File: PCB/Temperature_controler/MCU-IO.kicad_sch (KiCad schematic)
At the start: 14 parts, among them U1 STM32F401RBTx

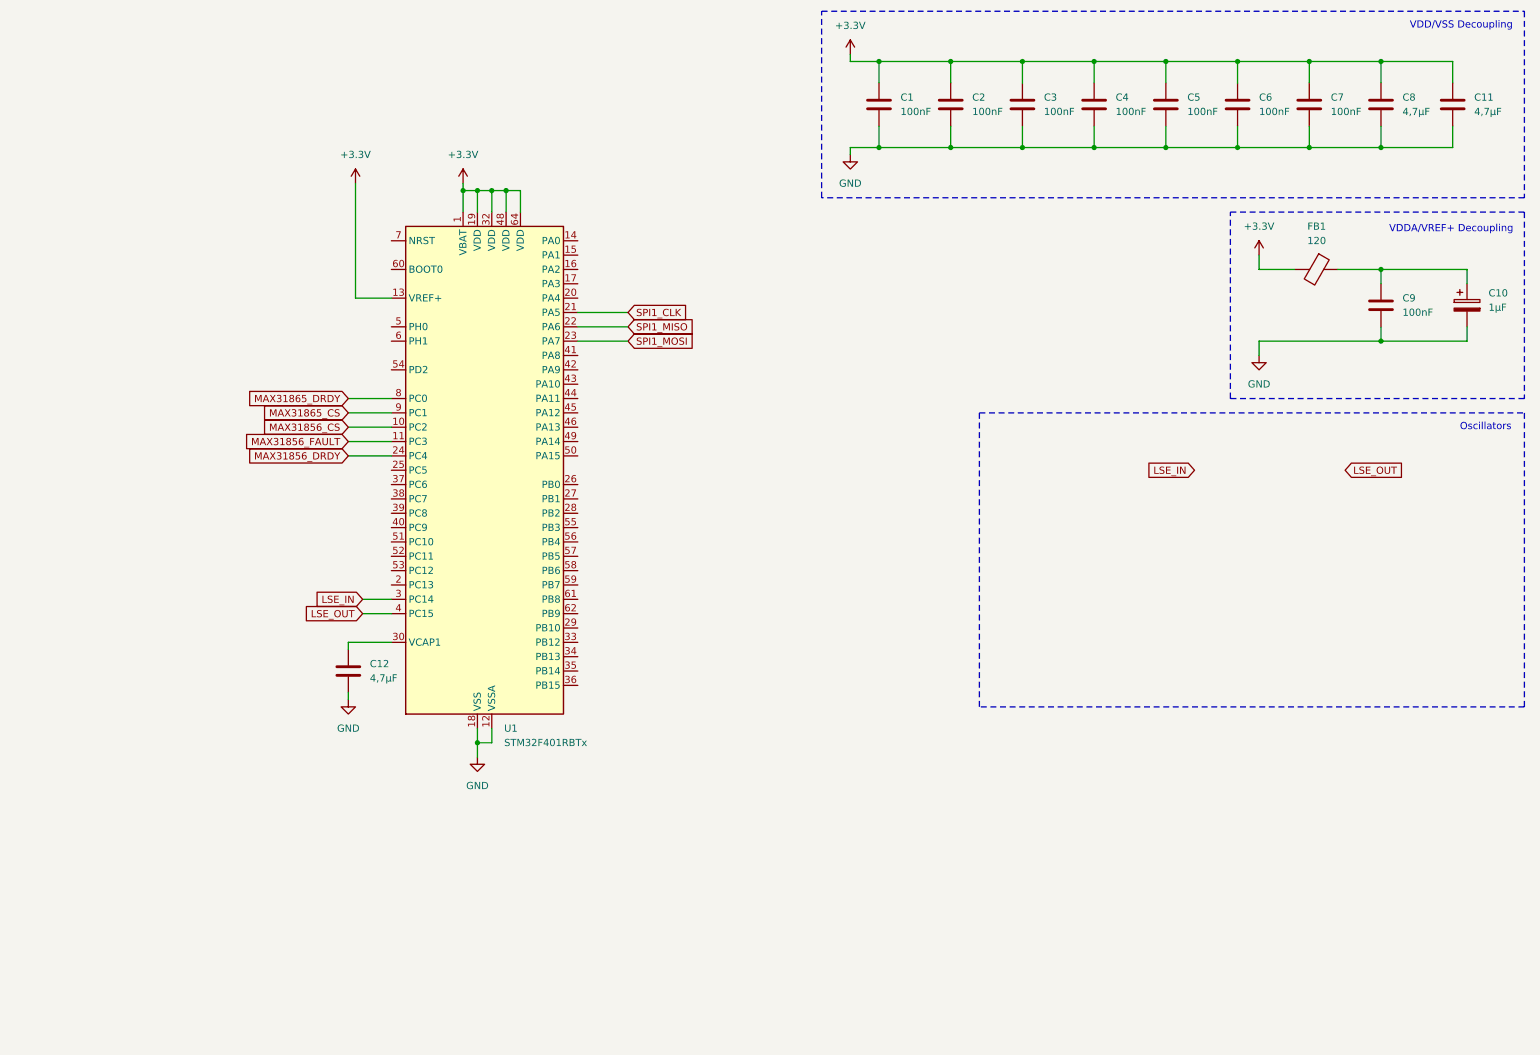
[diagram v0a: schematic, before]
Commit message: PCB progress
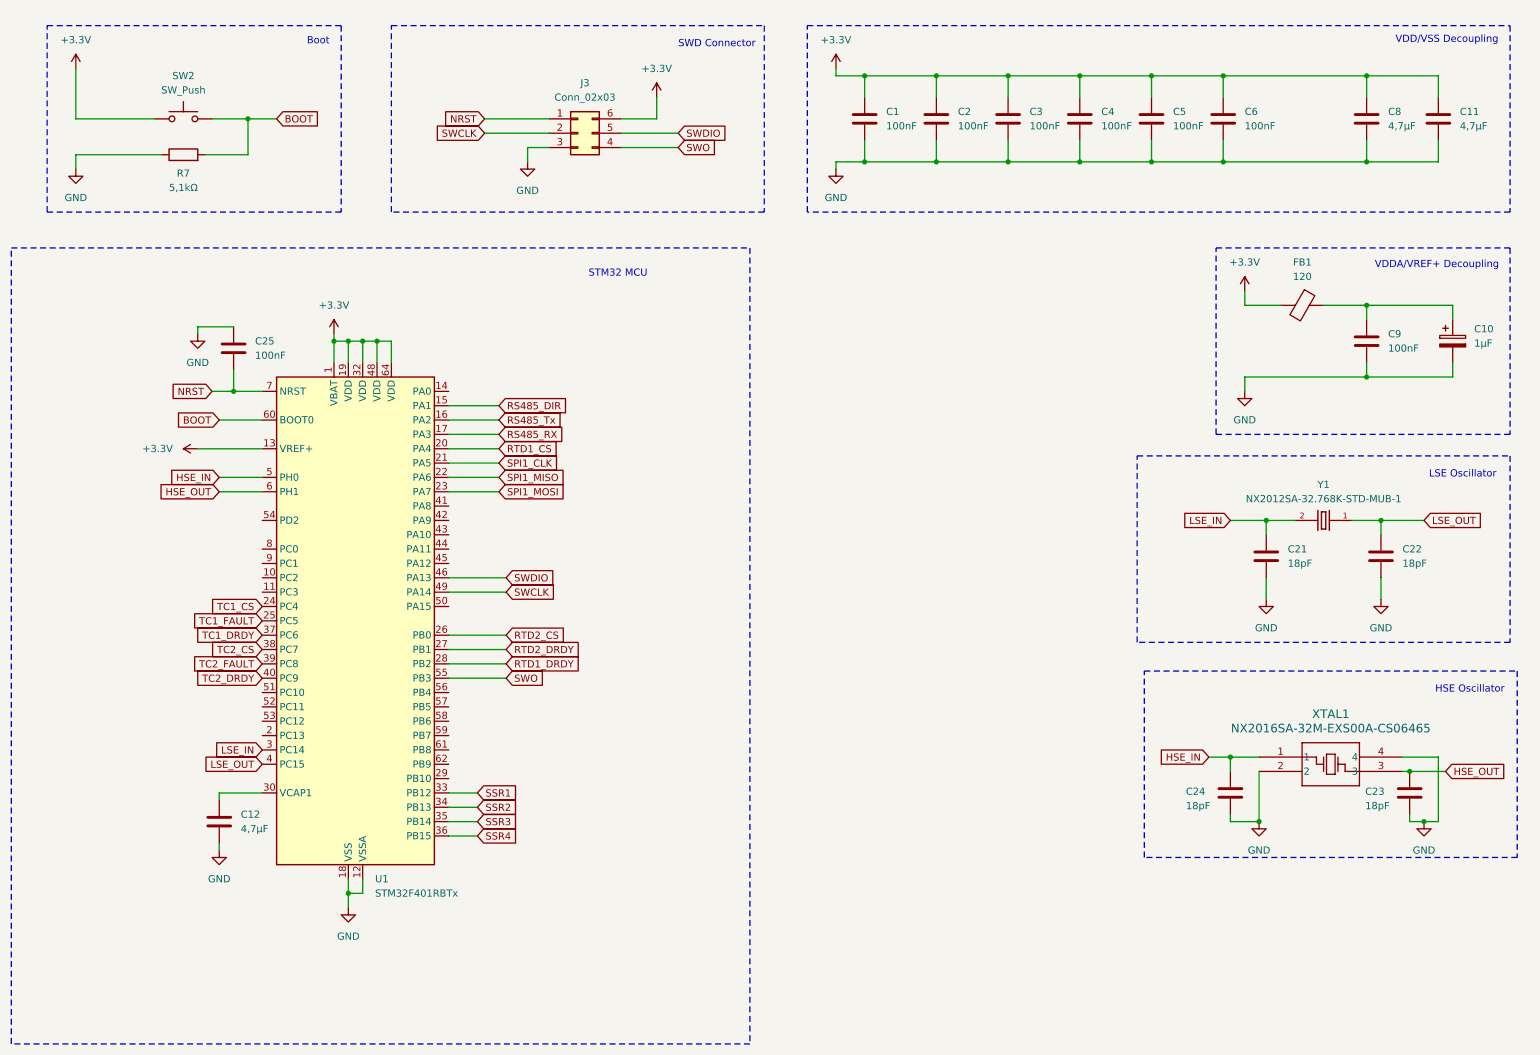
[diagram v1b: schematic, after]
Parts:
- removed C7: 100nF, symbol Device:C
- added C21, C22, C23, C24: 18pF, Capacitor_SMD:C_0805_2012Metric_Pad1.18x1.45mm_HandSolder, symbol Device:C
- added C25: 100nF, Capacitor_SMD:C_0805_2012Metric_Pad1.18x1.45mm_HandSolder, symbol Device:C
- added J3: Conn_02x03, Connector_RJ:RJ45_Amphenol_RJHSE538X, symbol Connector_Generic:Conn_02x03_Counter_Clockwise
- added R7: 5,1kΩ, Resistor_SMD:R_0805_2012Metric_Pad1.20x1.40mm_HandSolder, symbol Device:R
- added SW2: SW_Push, Button_Switch_SMD:SW_Push_1P1T-SH_NO_CK_KMR2xxG, symbol Switch:SW_Push
- added XTAL1: NX2016SA-32M-EXS00A-CS06465, NX2016SA-32M-EXS00A-CS06465:NX2016SA_NDK, symbol NX2016SA-32M-EXS00A-CS06465:NX2016SA-32M-EXS00A-CS06465
- added Y1: NX2012SA-32.768K-STD-MUB-1, NX2012SA-32.768K-STD-MUB-1:XTAL_NX2012SA-32.768K-STD-MUB-1, symbol NX2012SA-32.768K-STD-MUB-1:NX2012SA-32.768K-STD-MUB-1
- C1, C10, C11, C12, C2, C3, C4, C5, C6, C8, C9: footprint (none) -> Capacitor_SMD:C_0805_2012Metric_Pad1.18x1.45mm_HandSolder
- FB1: footprint (none) -> Fuse:Fuse_2010_5025Metric_Pad1.52x2.65mm_HandSolder
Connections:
- net +3.3V: now also J3.6 (Pin_6), SW2.1
- net GND: now also C21.2, C22.2, C23.2, C24.2, C25.1, J3.3 (Pin_3), R7.1, XTAL1.2, XTAL1.4
- net LSE_IN: now also C21.1, Y1.2
- net LSE_OUT: now also C22.1, Y1.1
- net RS485_DIR: now reaches U1.15 (PA1)
- net RS485_Tx: now reaches U1.16 (PA2)
- net RS485_RX: now reaches U1.17 (PA3)
- net RTD1_CS: now reaches U1.20 (PA4)
- net TC1_FAULT: now reaches U1.25 (PC5)
- net RTD2_CS: now reaches U1.26 (PB0)
- net RTD2_DRDY: now reaches U1.27 (PB1)
- net RTD1_DRDY: now reaches U1.28 (PB2)
- net SSR1: now reaches U1.33 (PB12)
- net SSR2: now reaches U1.34 (PB13)
- net SSR3: now reaches U1.35 (PB14)
- net SSR4: now reaches U1.36 (PB15)
- net TC1_DRDY: now reaches U1.37 (PC6)
- net TC2_CS: now reaches U1.38 (PC7)
- net TC2_FAULT: now reaches U1.39 (PC8)
- net TC2_DRDY: now reaches U1.40 (PC9)
- net SWDIO: now reaches U1.46 (PA13)
- net SWDIO: now also J3.5 (Pin_5)
- net SWCLK: now reaches U1.49 (PA14)
- net SWCLK: now also J3.2 (Pin_2)
- net HSE_IN: now reaches U1.5 (PH0)
- net HSE_IN: now also C24.1, XTAL1.1
- net SWO: now reaches U1.55 (PB3)
- net SWO: now also J3.4 (Pin_4)
- net HSE_OUT: now reaches U1.6 (PH1)
- net HSE_OUT: now also C23.1, XTAL1.3
- net BOOT: now reaches U1.60 (BOOT0)
- net BOOT: now also R7.2, SW2.2
- net NRST: now reaches U1.7 (NRST)
- net NRST: now also C25.2, J3.1 (Pin_1)
- net MAX31856_CS: no longer names the net of U1.10 (PC2)
- net MAX31856_DRDY renamed TC1_CS
- net MAX31856_FAULT: no longer names the net of U1.11 (PC3)
- net MAX31865_CS: no longer names the net of U1.9 (PC1)
- net MAX31865_DRDY: no longer names the net of U1.8 (PC0)
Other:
- note added: "Boot"
- note added: "HSE Oscillator"
- note added: "LSE Oscillator"
- note added: "STM32 MCU"
- note added: "SWD Connector"
- note removed: "Oscillators"
- moved on the sheet: C1, C10, C11, C12, C2, C3, C4, C5, C6, C8, C9, FB1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
